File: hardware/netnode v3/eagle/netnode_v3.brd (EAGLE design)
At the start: 59.9 x 58.9 mm, 25 parts, among them IC1 TSR-1, IC2 PIC18F4K80, X1 DC10R, X2 XPORT

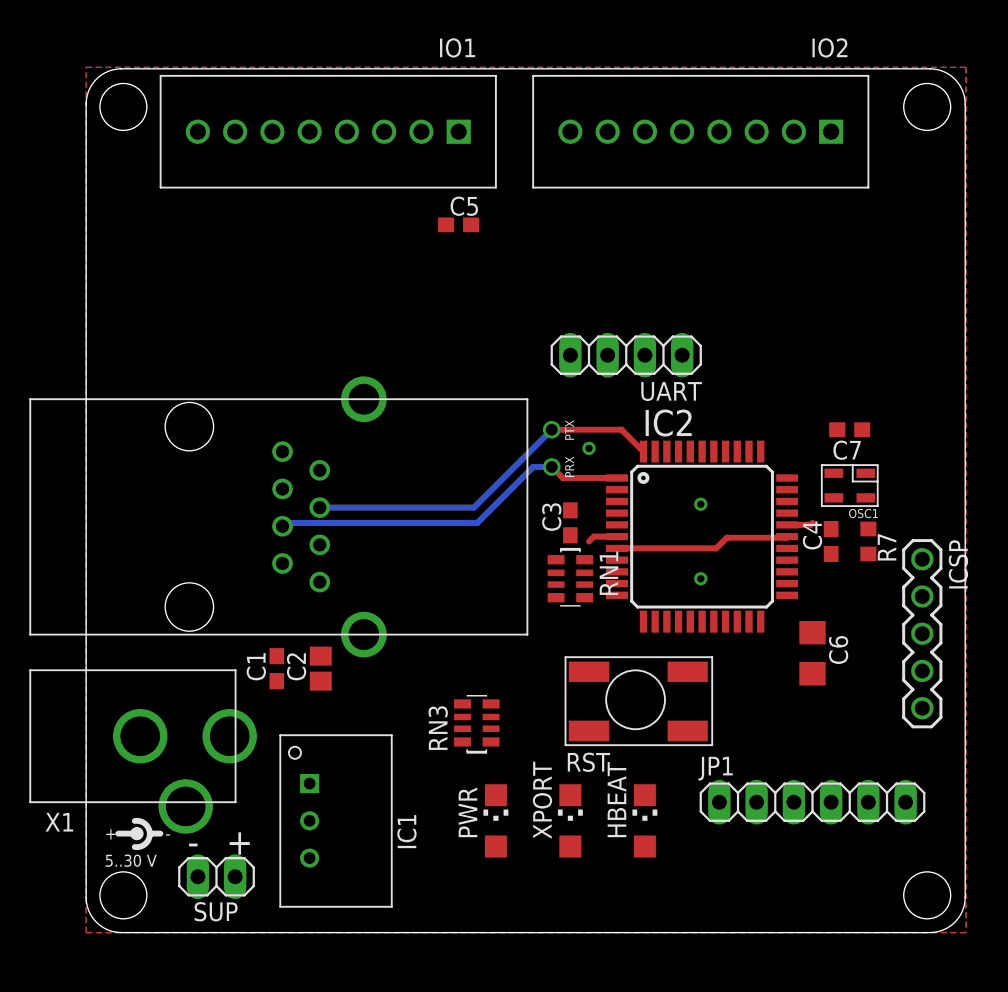
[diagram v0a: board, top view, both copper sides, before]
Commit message: Pre-final board files, silkscreen to be fixed
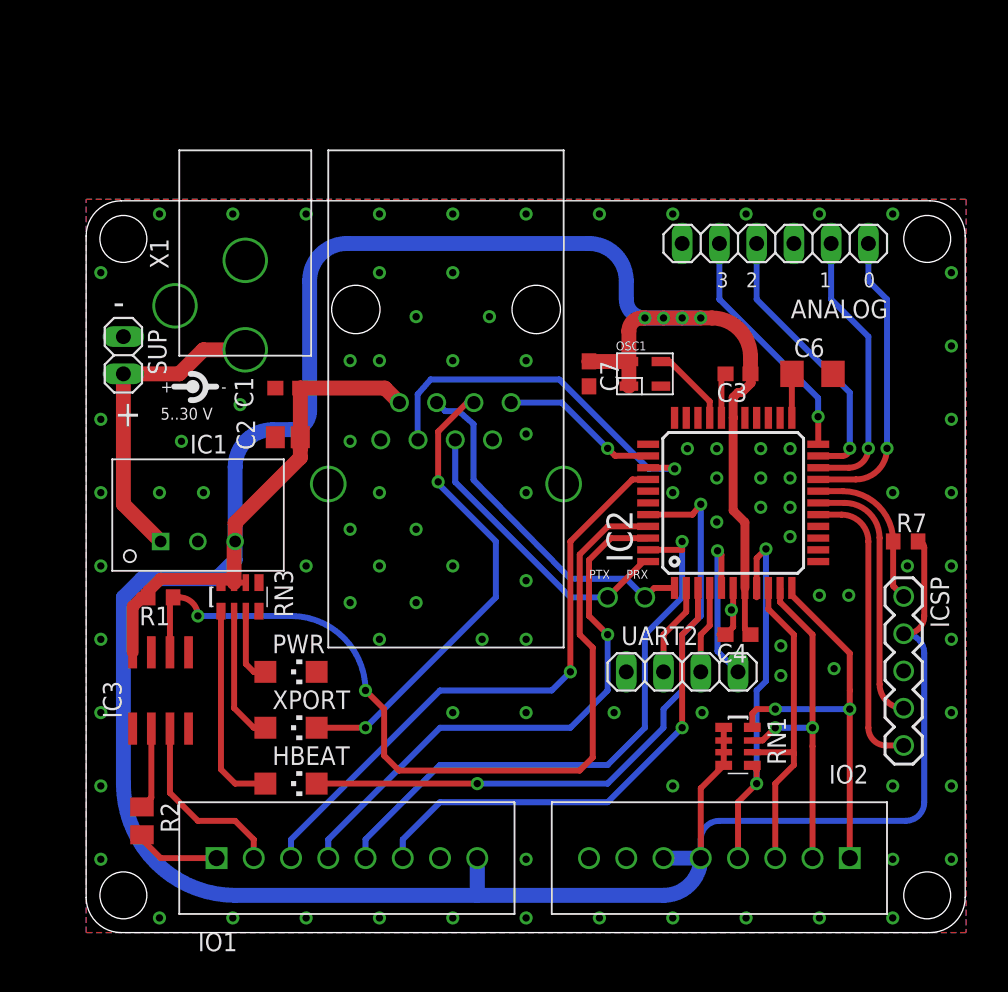
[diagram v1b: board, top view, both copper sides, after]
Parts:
- removed C5: 100n, rcl:C0603
- removed JP1: (no value), pinhead:1X06
- removed RST: 9902031, netnode:PUSHBUTTON
- removed UART: (no value), pinhead:1X04
- added ANALOG: (no value), pinhead:1X06
- added IC3: FOD060L, ic:SO-08
- added R1: 2K, rcl:R0603
- added R2: (no value), rcl:M0805
- added UART2: (no value), pinhead:1X04
- moved IO1 52.2 mm to (8.89, 5.08), turned to 0 degrees
- moved IO2 49.5 mm to (52.1, 5.08)
- moved X1 45.6 mm to (6.35, 53.3), turned to 270 degrees
- moved X2 38.8 mm to (16.5, 53.3), turned to 270 degrees
- moved SUP 36.1 mm to (2.54, 39.4), turned to 270 degrees
- moved HBEAT 24.3 mm to (14.0, 10.2), turned to 270 degrees
- moved XPORT 20.1 mm to (14.0, 14.0), turned to 270 degrees
- moved IC1 19.4 mm to (5.08, 26.7), turned to 0 degrees
- moved C1 19.1 mm to (13.8, 37.1), turned to 180 degrees
- moved C6 19.1 mm to (49.5, 38.1), turned to 0 degrees
- moved RN3 18.3 mm to (10.5, 22.9), turned to 0 degrees
- moved C7 18.2 mm to (34.3, 38.1), turned to 270 degrees
- moved PWR 17.3 mm to (14.0, 17.8), turned to 270 degrees
- moved RN1 16.2 mm to (44.5, 12.7)
- moved C2 15.9 mm to (13.8, 33.8), turned to 180 degrees
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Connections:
- removed net N$12: IC2.2, UART.2
- removed net N$9: HBEAT.C, IC2.15
- new net HBEAT: HBEAT.C, IC2.40
- new net N$3: IO1.1, R2.2
- new net OPTO1: IC2.41, IC3.6, R1.1
- new net RD4: IC2.2, UART2.2
- net !MCLR: no longer RST.3
- net +3V3: now also IC3.8, IO1.8, IO2.5, IO2.6, R1.2, RN3.6; no longer C5.1, IO1.1, RN3.5
- net AN0: now also ANALOG.1; no longer JP1.1
- net AN1: now also ANALOG.2; no longer JP1.2
- net AN2: now also ANALOG.4; no longer JP1.4
- net AN3: now also ANALOG.5; no longer JP1.5
- net GND: now also ANALOG.3, ANALOG.6, IC3.5, IO1.7, IO2.7, UART2.1; no longer C5.2, IO1.2, IO2.2, IO2.4, IO2.6, JP1.3, JP1.6, RST.1, UART.1
- net IN0: now also IO2.4, RN1.5; no longer IO2.1, RN1.8
- net IN1: now also RN1.6; no longer RN1.7
- net IN2: now also IO2.2, RN1.7; no longer IO2.5, RN1.6
- net IN3: now also IO2.1, RN1.8; no longer IO2.7, RN1.5
- net N$2: now also RN3.3; no longer RN3.1
- net N$8: now also RN3.1; no longer RN3.4
- net OPTO+: now also IC3.2, R2.1; no longer IO1.5
- net OPTO-: now also IC3.3, IO1.2; no longer IO1.6
- net OW: now also IO1.5; no longer IO1.7
- net PIC_RTS: now also IC2.35
- net PWM: now also IO1.6; no longer IO1.8
- net RX2: now also UART2.4; no longer UART.4
- net TX2: now also UART2.3; no longer UART.3
- net XPORT_RST: now also IC2.36
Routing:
- net +3V3: track 11.9 -> 241.2 mm, vias 0 -> 4
- net OPTO1: track 0.00 -> 59.2 mm, vias 0 -> 2
- net HBEAT: track 0.00 -> 45.5 mm, vias 0 -> 2
- net SCL: track 0.00 -> 41.0 mm, vias 0 -> 1
- net OW: track 0.00 -> 40.1 mm, vias 0 -> 1
- net SDA: track 0.00 -> 38.6 mm, vias 0 -> 1
- net PWM: track 0.00 -> 33.5 mm, vias 0 -> 1
- net XPORT_STAT: track 0.00 -> 32.1 mm, vias 0 -> 2
- net IN3: track 0.00 -> 27.8 mm, vias 0 -> 2
- net IN0: track 0.00 -> 26.8 mm, vias 0 -> 2
- net XPORT_RST: track 0.00 -> 25.5 mm, vias 0 -> 1
- net IN2: track 0.00 -> 23.8 mm, vias 0 -> 2
- net IN1: track 0.00 -> 22.5 mm
- net VSUPPLY: track 0.00 -> 21.5 mm
- net AN0: track 0.00 -> 20.1 mm, vias 0 -> 1
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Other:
- board size 59.9 x 58.9 mm -> 59.9 x 49.9 mm
- board text added: "0"
- board text added: "1"
- board text added: "2"
- board text added: "3"
